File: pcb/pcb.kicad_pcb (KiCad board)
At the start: 2 copper layers, 34 parts, among them J1 Conn_02x08_Odd_Even, J2 B2B-PH-K-S_LF__SN_, J3 USB_C_Receptacle, Q1 MMUN2211LT1G, SW1 SW_SPST, U1 TPS61090, U2 MCP73871-1AA

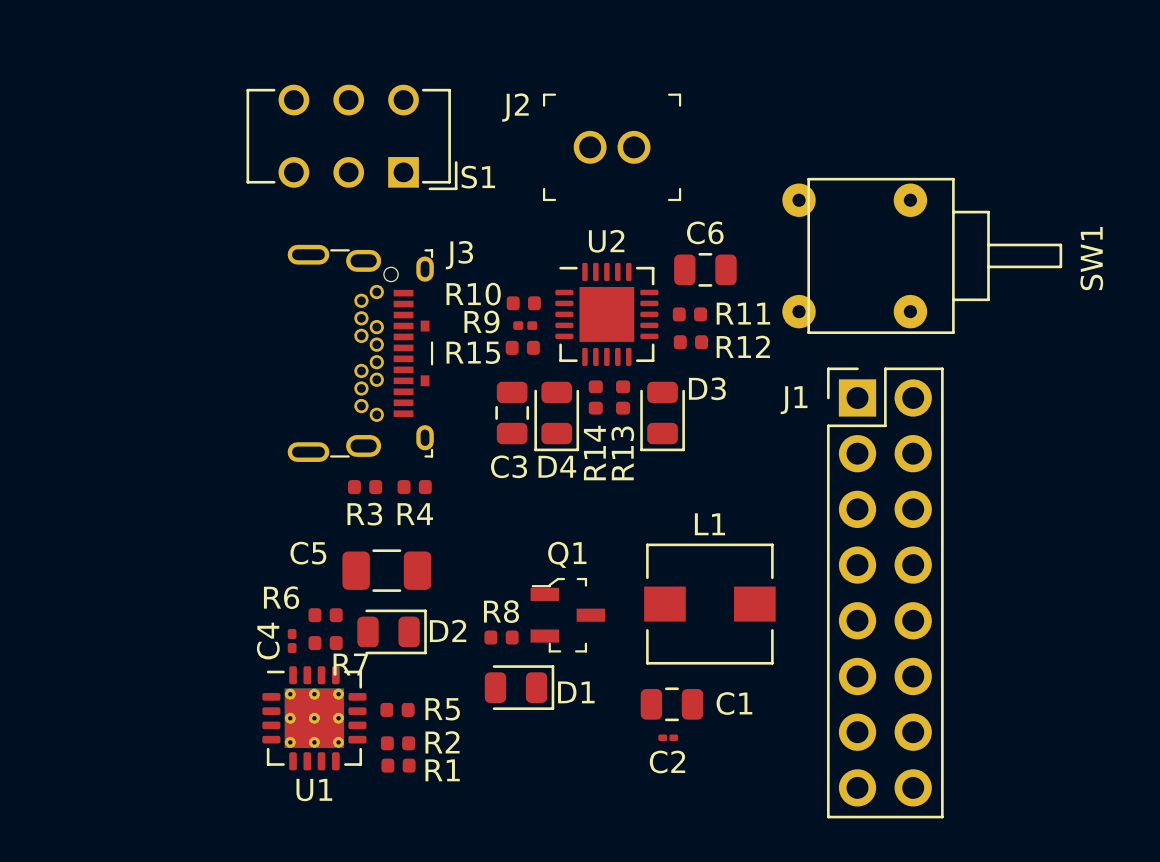
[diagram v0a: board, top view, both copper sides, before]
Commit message: in work, PCB layup
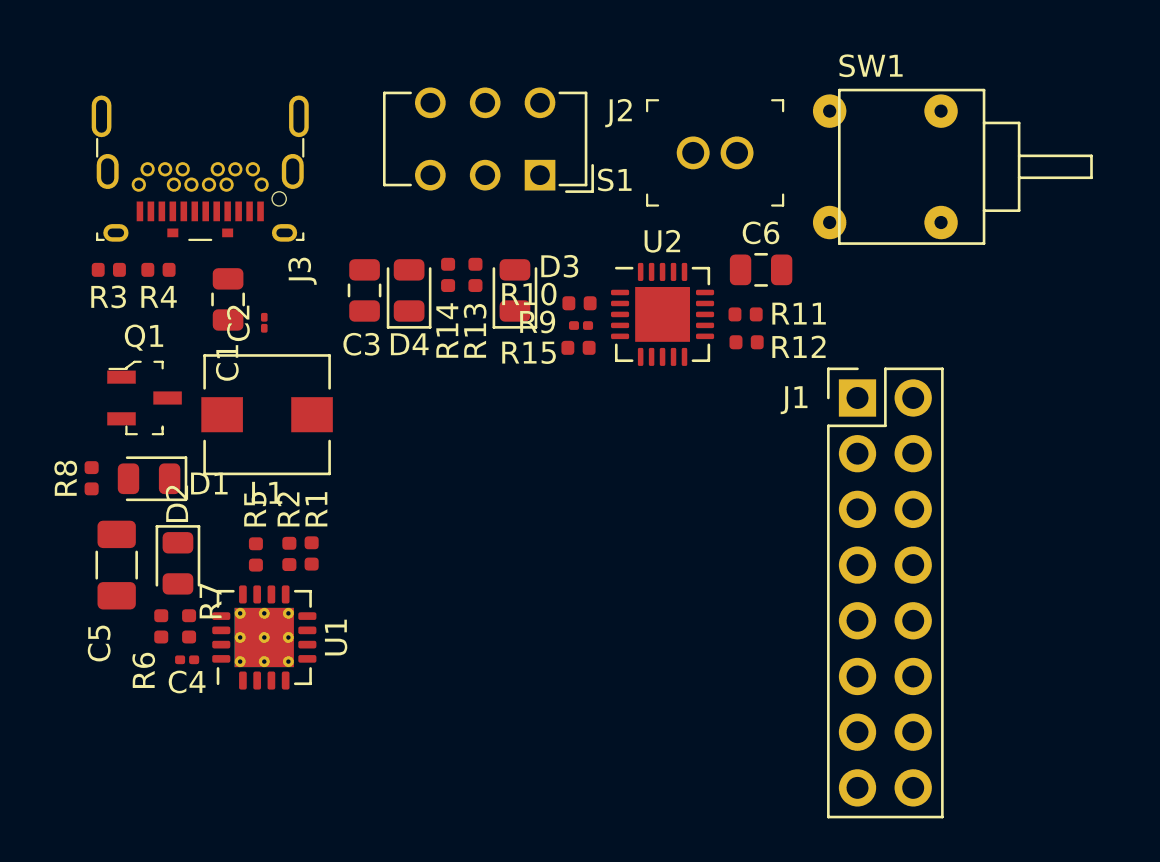
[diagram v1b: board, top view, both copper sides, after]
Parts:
- moved C1 27.4 mm to (183.4, 90.8), turned to 270 degrees
- moved C2 26.4 mm to (185.0, 91.8), turned to 270 degrees
- moved L1 22.0 mm to (185.2, 96.0), turned to 180 degrees
- moved Q1 21.7 mm to (179.6, 95.2)
- moved R8 20.1 mm to (177.2, 98.9), turned to 270 degrees
- moved D1 19.3 mm to (179.8, 98.9)
- moved R3 15.3 mm to (177.9, 89.4)
- moved R4 15.3 mm to (180.2, 89.4)
- moved C5 12.3 mm to (178.3, 102.9), turned to 90 degrees
- moved J3 11.3 mm to (182.1, 86.7), turned to 180 degrees
- moved R1 10.5 mm to (187.2, 102.3), turned to 270 degrees
- moved D2 10.1 mm to (181.1, 102.8), turned to 270 degrees
- moved R2 9.96 mm to (186.2, 102.4), turned to 90 degrees
- moved R5 9.59 mm to (184.7, 102.4), turned to 270 degrees
- moved C3 8.75 mm to (189.6, 90.3)
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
